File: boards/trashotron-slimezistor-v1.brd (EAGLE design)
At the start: 76.2 x 76.2 mm, 17 parts, among them IC1 2967-MP6500, IC2 2967-MP6500, IC3 2967-MP6500, J4 455-1750-1-ND, J6 455-1750-1-ND, J9 455-1750-1-ND, U2 LM358

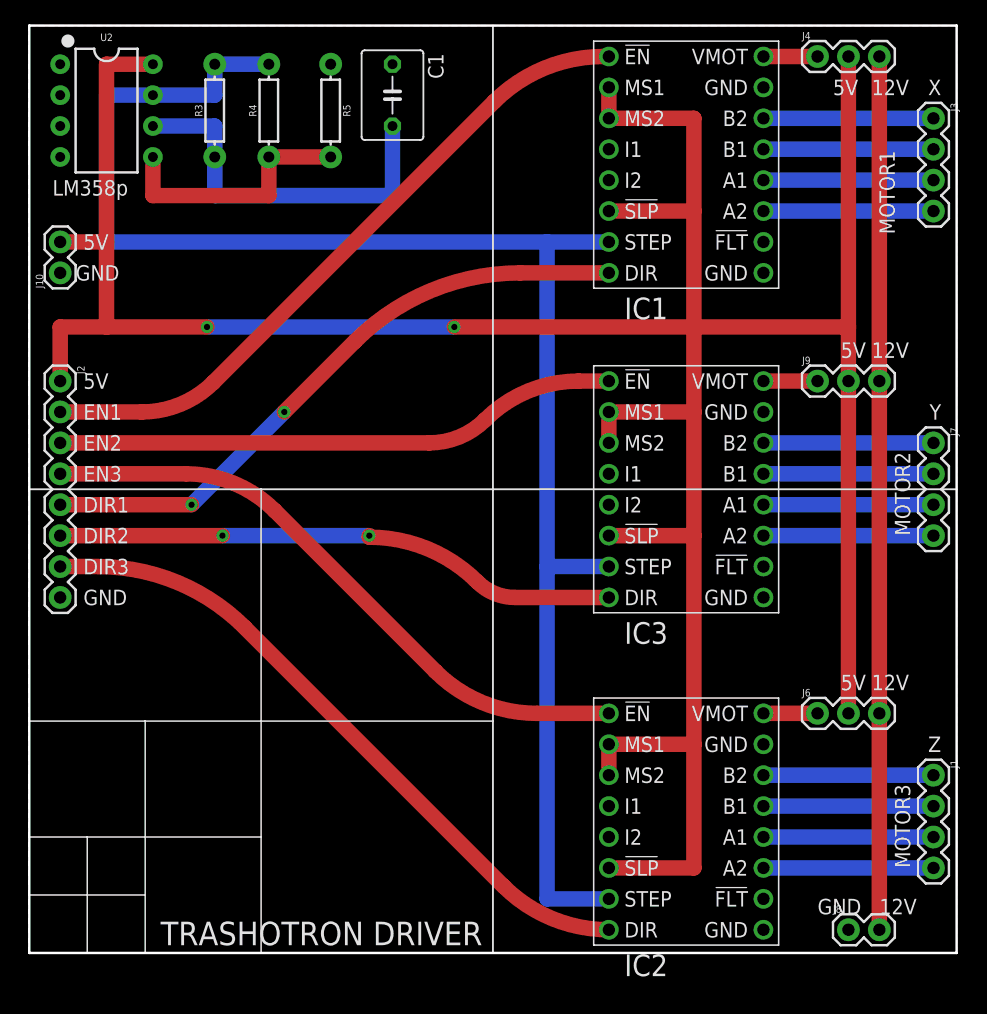
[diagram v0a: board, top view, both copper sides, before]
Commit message: lots of work on pcb layout
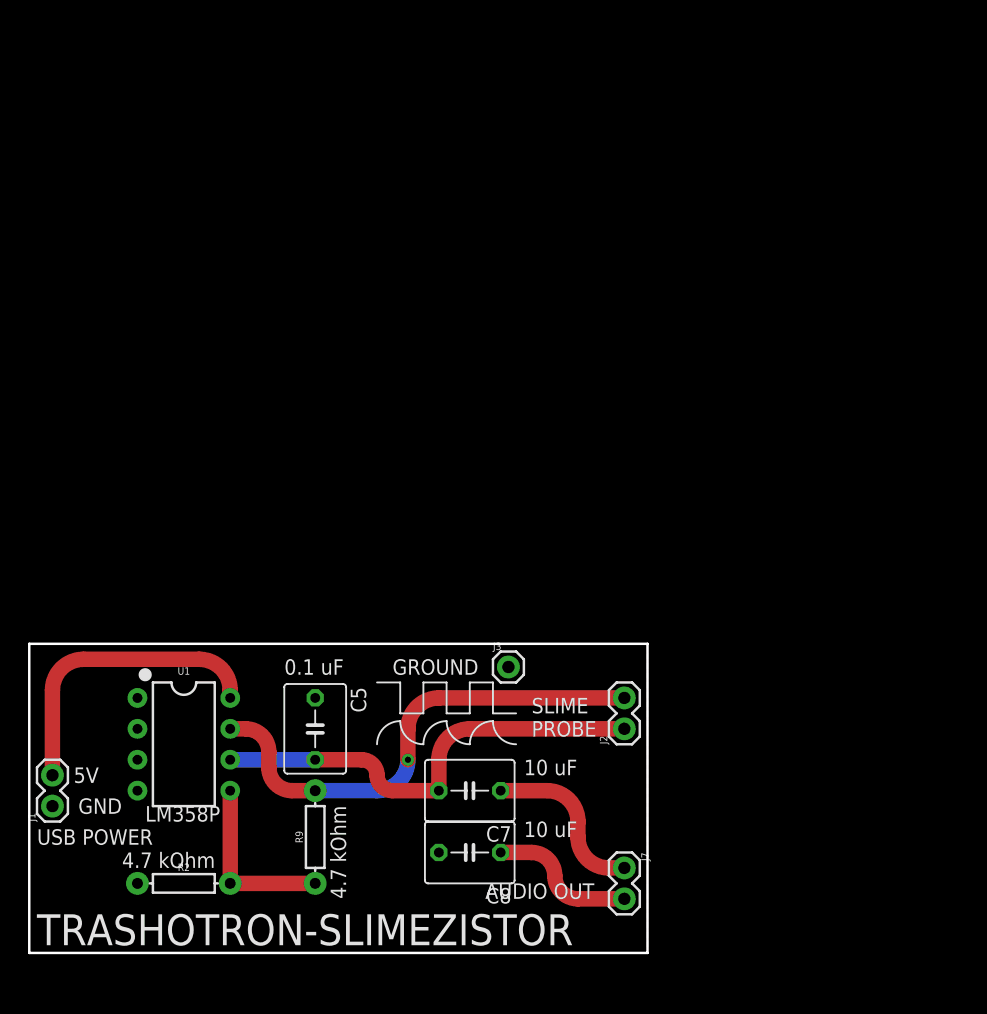
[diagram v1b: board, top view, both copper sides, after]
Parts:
- removed C1: (no value), rcl:C050-050X075
- removed IC1, IC2, IC3: 2967-MP6500, pololu-stepper-driver:MP6500
- removed J10, J8: (no value), SparkFun-Connectors:1X02
- removed J4, J6, J9: 455-1750-1-ND, SparkFun-Connectors:1X03
- removed R3, R4, R5: (no value), SparkFun-Resistors:AXIAL-0.3
- removed U2: LM358, SparkFun-IC-Amplifiers:DIP08
- added C5, C7, C8: (no value), rcl:C050-050X075
- added R2, R9: (no value), SparkFun-Resistors:AXIAL-0.3
- added U1: LM358, SparkFun-IC-Amplifiers:DIP08
- J1, J7: device SparkFun-Connectors:1X04 -> SparkFun-Connectors:1X02
- J2: device SparkFun-Connectors:1X08 -> SparkFun-Connectors:1X02
- J3: device SparkFun-Connectors:1X04 -> SparkFun-Connectors:1X01
- moved J1 72.4 mm to (1.91, 12.1), turned to 90 degrees
- moved J3 57.0 mm to (39.4, 23.5), turned to 0 degrees
- moved J2 54.5 mm to (48.9, 18.4), turned to 90 degrees
- moved J7 43.2 mm to (48.9, 6.99)
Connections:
- removed net 5V: IC1.2, IC1.3, IC1.6, IC2.2, IC2.3, IC2.6, IC3.2, IC3.3, IC3.6, J10.2, J2.1, J4.2, J6.2, J9.2, U2.8
- removed net CLOCK: IC1.7, IC2.7, IC3.7, R3.P$2, R4.P$2, U2.7
- removed net DIR1: IC1.8, J2.5
- removed net DIR2: IC3.8, J2.6
- removed net DIR3: IC2.8, J2.7
- removed net EN1: IC1.1, J2.2
- removed net EN2: IC3.1, J2.3
- removed net EN3: IC2.1, J2.4
- removed net EXTPOW: J4.3, J6.3, J8.2, J9.3
- removed net N$1: IC3.14, J7.1
- removed net N$11: IC2.12, J1.3
- removed net N$13: IC3.12, J7.3
- removed net N$18: C1.2, R3.P$1, U2.6
- removed net N$19: R4.P$1, R5.P$2, U2.5
- removed net N$4: IC3.13, J7.2
- removed net N$6: IC1.13, J3.2
- removed net N$7: IC1.12, J3.3
- removed net N$8: IC1.11, J3.4
- removed net N$9: IC2.14, J1.1
- removed net VMOT1: IC1.16, J4.1
- removed net VMOT2: IC3.16, J9.1
- removed net VMOT3: IC2.16, J6.1
- new net N$16: C7.1, J7.1
- new net VCC: J1.2, U1.8
- net GND: now also C5.1, C8.2, J1.1, J3.1, R2.P$1, U1.4; no longer C1.1, IC1.15, IC1.9, IC2.15, IC2.9, IC3.15, IC3.9, J10.1, J2.8, J8.1, R5.P$1, U2.4
- net N$10: now also R2.P$2, R9.P$1, U1.5; no longer IC2.13, J1.2
- net N$12: now also C5.2, C7.2, J2.1, U1.6; no longer IC2.11, J1.4
- net N$14: now also C8.1, J7.2; no longer IC3.11, J7.4
- net N$5: now also J2.2, R9.P$2, U1.7; no longer IC1.14, J3.1
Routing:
- net 5V: track 263.5 -> 0.00 mm, vias 2 -> 0
- net CLOCK: track 133.3 -> 0.00 mm
- net EXTPOW: track 71.8 -> 0.00 mm
- net EN1: track 55.9 -> 0.00 mm
- net DIR3: track 55.6 -> 0.00 mm
- net EN3: track 51.8 -> 0.00 mm
- net DIR1: track 51.8 -> 0.00 mm, vias 2 -> 0
- net DIR2: track 46.2 -> 0.00 mm, vias 2 -> 0
- net EN2: track 46.1 -> 0.00 mm
- net N$18: track 31.1 -> 0.00 mm
- net N$5: track 14.0 -> 39.9 mm, vias 0 -> 1
- net VCC: track 0.00 -> 24.3 mm
- net N$12: track 14.0 -> 37.0 mm
- net N$19: track 21.0 -> 0.00 mm
- net N$9: track 14.0 -> 0.00 mm
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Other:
- board size 76.2 x 76.2 mm -> 50.8 x 25.4 mm
- board text added: "0.1 uF"
- board text added: "10 uF"
- board text added: "4.7 kOhm"
- board text added: "AUDIO OUT"
- board text added: "GROUND"
- board text added: "LM358P"
- board text added: "SLIME PROBE"
- board text added: "TRASHOTRON-SLIMEZISTOR"
- board text added: "USB POWER"
- board text removed: "12V"
- board text removed: "DIR1"
- board text removed: "DIR2"
- board text removed: "DIR3"
- board text removed: "EN1"
- board text removed: "EN2"
- board text removed: "EN3"
- board text removed: "LM358p"
- board text removed: "MOTOR1"
- board text removed: "MOTOR2"
- board text removed: "MOTOR3"
- board text removed: "TRASHOTRON DRIVER"
- board text removed: "X"
- board text removed: "Y"
- board text removed: "Z"
